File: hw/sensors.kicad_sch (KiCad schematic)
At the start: 40 parts, among them IC2 INA215CQDCKRQ1, IC5 OPA990IDCKR, IC6 INA215CQDCKRQ1, U5 MAX31865xTP, U6 ADG734

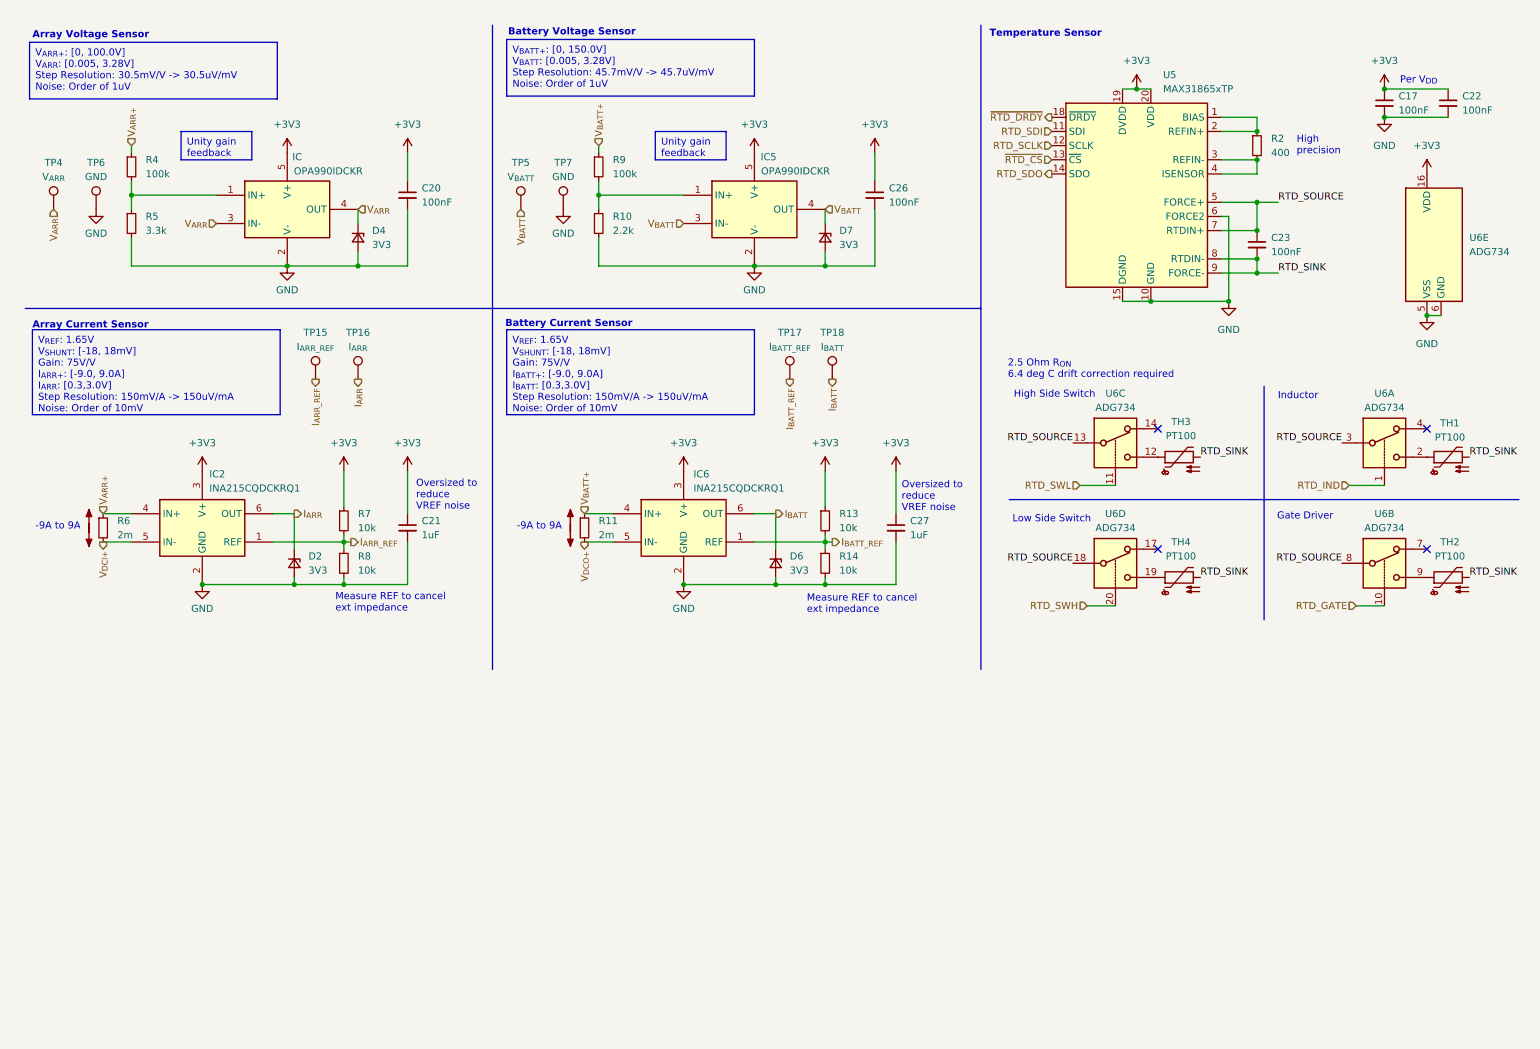
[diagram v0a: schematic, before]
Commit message: v0.3.0rc (v1.0.0rc) sch complete
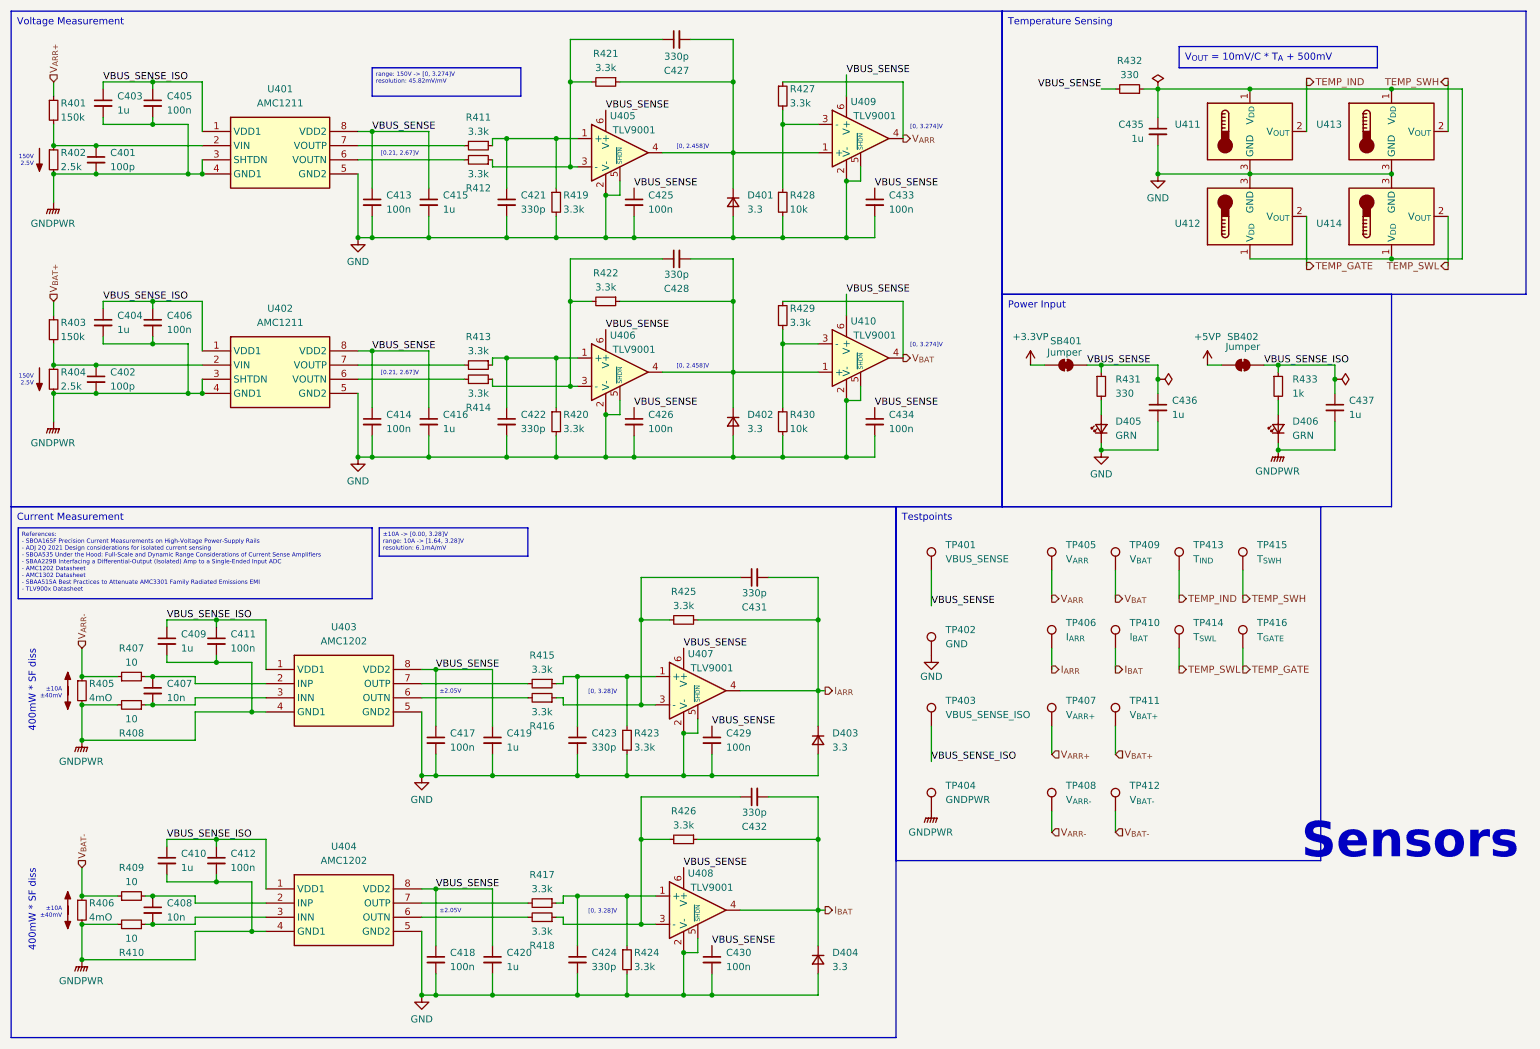
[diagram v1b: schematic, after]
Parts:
- removed C17, C20, C22, C23, C26: 100nF, symbol Device:C_Small
- removed C21, C27: 1uF, symbol Device:C_Small
- removed D2, D4, D6, D7: 3V3, Diode_SMD:D_MiniMELF, symbol Device:D_Zener_Small
- removed IC, IC5: OPA990IDCKR, footprints:ti_OPA990IDCKR, symbol ti_OPA990IDCKR:OPA990IDCKR
- removed IC2, IC6: INA215CQDCKRQ1, footprints:ti_INA215CQDCKRQ1, symbol ti_INA215CQDCKRQ1:INA215CQDCKRQ1
- removed R10: 2.2k, symbol Device:R_Small
- removed R11, R6: 2m, symbol Device:R_Small
- removed R13, R14, R7, R8: 10k, symbol Device:R_Small
- removed R2: 400, symbol Device:R_Small
- removed R4, R9: 100k, symbol Device:R_Small
- removed R5: 3.3k, symbol Device:R_Small
- removed TH1, TH2, TH3, TH4: PT100, symbol Sensor_Temperature:PT100
- removed TP15: I_{ARR_REF}, symbol Connector:TestPoint
- removed TP16: I_{ARR}, symbol Connector:TestPoint
- removed TP17: I_{BATT_REF}, symbol Connector:TestPoint
- removed TP18: I_{BATT}, symbol Connector:TestPoint
- removed TP4: V_{ARR}, symbol Connector:TestPoint
- removed TP5: V_{BATT}, symbol Connector:TestPoint
- removed TP6, TP7: GND, symbol Connector:TestPoint
- removed U5: MAX31865xTP, Package_DFN_QFN:TQFN-20-1EP_5x5mm_P0.65mm_EP3.25x3.25mm, symbol Sensor_Temperature:MAX31865xTP
- removed U6: ADG734, Package_SO:TSSOP-20_4.4x6.5mm_P0.65mm, symbol Analog_Switch:ADG734
- added C401, C402: 100p, Resistor_SMD:R_0402_1005Metric, symbol Device:C_Small
- added C403, C404, C409, C410, C415, C416, C419, C420, C435, C436, C437: 1u, Resistor_SMD:R_0402_1005Metric, symbol Device:C_Small
- added C405, C406, C411, C412, C413, C414, C417, C418, C425, C426, C429, C430, C433, C434: 100n, Resistor_SMD:R_0402_1005Metric, symbol Device:C_Small
- added C407, C408: 10n, Resistor_SMD:R_0402_1005Metric, symbol Device:C_Small
- added C421, C422, C423, C424, C427, C428, C431, C432: 330p, Resistor_SMD:R_0402_1005Metric, symbol Device:C_Small
- added D401, D402, D403, D404: 3.3, Diode_SMD:D_SOD-123, symbol Device:D_Small
- added D405, D406: GRN, LED_SMD:LED_0402_1005Metric, symbol Device:LED_Small
- added R401, R403: 150k, Resistor_SMD:R_0805_2012Metric, symbol Device:R_Small
- added R402, R404: 2.5k, Resistor_SMD:R_0805_2012Metric, symbol Device:R_Small
- added R405, R406: 4mO, Resistor_SMD:R_2512_6332Metric, symbol Device:R_Small
- added R407, R408, R409, R410: 10, Resistor_SMD:R_0402_1005Metric, symbol Device:R_Small
- added R411, R412, R413, R414, R415, R416, R417, R418, R419, R420, R421, R422, R423, R424, R425, R426, R427, R429: 3.3k, Resistor_SMD:R_0402_1005Metric, symbol Device:R_Small
- added R428, R430: 10k, Resistor_SMD:R_0402_1005Metric, symbol Device:R_Small
- added R431, R432: 330, Resistor_SMD:R_0402_1005Metric, symbol Device:R_Small
- added R433: 1k, Resistor_SMD:R_0402_1005Metric, symbol Device:R_Small
- added SB401, SB402: Jumper, Jumper:SolderJumper-2_P1.3mm_Open_TrianglePad1.0x1.5mm, symbol Jumper:SolderJumper_2_Bridged
- added TP401: VBUS_SENSE, TestPoint:TestPoint_Keystone_5000-5004_Miniature, symbol Connector:TestPoint
- added TP402: GND, TestPoint:TestPoint_Keystone_5000-5004_Miniature, symbol Connector:TestPoint
- added TP403: VBUS_SENSE_ISO, TestPoint:TestPoint_Keystone_5000-5004_Miniature, symbol Connector:TestPoint
- added TP404: GNDPWR, TestPoint:TestPoint_Keystone_5000-5004_Miniature, symbol Connector:TestPoint
- added TP405: V_{ARR}, TestPoint:TestPoint_Keystone_5000-5004_Miniature, symbol Connector:TestPoint
- added TP406: I_{ARR}, TestPoint:TestPoint_Keystone_5000-5004_Miniature, symbol Connector:TestPoint
- added TP407: V_{ARR+}, TestPoint:TestPoint_Keystone_5000-5004_Miniature, symbol Connector:TestPoint
- added TP408: V_{ARR-}, TestPoint:TestPoint_Keystone_5000-5004_Miniature, symbol Connector:TestPoint
- added TP409: V_{BAT}, TestPoint:TestPoint_Keystone_5000-5004_Miniature, symbol Connector:TestPoint
- added TP410: I_{BAT}, TestPoint:TestPoint_Keystone_5000-5004_Miniature, symbol Connector:TestPoint
- added TP411: V_{BAT+}, TestPoint:TestPoint_Keystone_5000-5004_Miniature, symbol Connector:TestPoint
- added TP412: V_{BAT-}, TestPoint:TestPoint_Keystone_5000-5004_Miniature, symbol Connector:TestPoint
- added TP413: T_{IND}, TestPoint:TestPoint_Keystone_5000-5004_Miniature, symbol Connector:TestPoint
- added TP414: T_{SWL}, TestPoint:TestPoint_Keystone_5000-5004_Miniature, symbol Connector:TestPoint
- added TP415: T_{SWH}, TestPoint:TestPoint_Keystone_5000-5004_Miniature, symbol Connector:TestPoint
- added TP416: T_{GATE}, TestPoint:TestPoint_Keystone_5000-5004_Miniature, symbol Connector:TestPoint
- added U401, U402: AMC1211, footprints:ti_AMC1211_DWV, symbol ti_AMC1211:AMC1211AQDWVRQ1
- added U403, U404: AMC1202, footprints:ti_AMC1202_DWV, symbol ti_AMC1202:AMC1202DWVR
- added U405, U406, U407, U408, U409, U410: TLV9001, Package_TO_SOT_SMD:SOT-363_SC-70-6, symbol ti_TLV9001:TLV9001
- added U411, U412, U413, U414: MCP9700A, Connector_JST:JST_PH_B3B-PH-K_1x03_P2.00mm_Vertical, symbol Sensor_Temperature:MCP9700Ax-ELT
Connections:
- net GND: now also C413.2, C414.2, C415.2, C416.2, C417.2, C418.2, C419.2, C420.2, C421.2, C422.2, C423.2, C424.2, C425.2, C426.2, C429.2, C430.2, C433.2, C434.2, C435.2, C436.2, D401.2 (A), D402.2 (A), D403.2 (A), D404.2 (A), D405.1 (K), R419.2, R420.2, R423.2, R424.2, R428.2, R430.2, TP402.1, U401.5 (GND2), U402.5 (GND2), U403.5 (GND2), U404.5 (GND2), U405.2 (V-), U405.5 (~{SHDN}), U406.2 (V-), U406.5 (~{SHDN}), U407.2 (V-), U407.5 (~{SHDN}), U408.2 (V-), U408.5 (~{SHDN}), U409.2 (V-), U409.5 (~{SHDN}), U410.2 (V-), U410.5 (~{SHDN}), U411.3 (GND), U412.3 (GND), U413.3 (GND), U414.3 (GND)
- net I_{ARR}: now also C431.2, D403.1 (K), R425.1, TP406.1, U407.4
- net V_{ARR+}: now also R401.1, TP407.1
- net V_{ARR}: now also R427.1, TP405.1, U409.4
- new net: C424.1, R417.1, R424.1, U408.1 (+)
- new net: C432.1, R418.1, R426.2, U408.3 (-)
- new net: C423.1, R415.1, R423.1, U407.1 (+)
- new net: C431.1, R416.1, R425.2, U407.3 (-)
- new net: C428.1, R414.1, R422.2, U406.3 (-)
- new net: R414.2, U402.6 (VOUTN)
- new net: C407.2, R408.1, U403.3 (INN)
- new net: R416.2, U403.6 (OUTN)
- new net: C427.2, D401.1 (K), R421.1, U405.4, U409.1 (+)
- new net: C421.1, R411.1, R419.1, U405.1 (+)
- new net: D406.2 (A), R433.2
- new net: C428.2, D402.1 (K), R422.1, U406.4, U410.1 (+)
- new net: R429.2, R430.1, U410.3 (-)
- new net: C402.1, R403.2, R404.1, U402.2 (VIN)
- new net: C427.1, R412.1, R421.2, U405.3 (-)
- new net: C407.1, R407.2, U403.2 (INP)
- new net: R415.2, U403.7 (OUTP)
- new net: C422.1, R413.1, R420.1, U406.1 (+)
- new net: D405.2 (A), R431.2
- new net: R427.2, R428.1, U409.3 (-)
- new net: C408.2, R410.1, U404.3 (INN)
- new net: C401.1, R401.2, R402.1, U401.2 (VIN)
- new net: R418.2, U404.6 (OUTN)
- new net: C435.1, R432.1, U411.1 (V_{DD}), U412.1 (V_{DD}), U413.1 (V_{DD}), U414.1 (V_{DD})
- new net: R413.2, U402.7 (VOUTP)
- new net: C408.1, R409.2, U404.2 (INP)
- new net: R417.2, U404.7 (OUTP)
- new net: R412.2, U401.6 (VOUTN)
- new net: R411.2, U401.7 (VOUTP)
- new net +3.3VP: SB401.1 (A)
- new net +5VP: SB402.1 (A)
- new net GNDPWR: C401.2, C402.2, C403.2, C404.2, C405.2, C406.2, C409.2, C410.2, C411.2, C412.2, C437.2, D406.1 (K), R402.2, R404.2, R405.2, R406.2, R408.2, R410.2, TP404.1, U401.3 (SHTDN), U401.4 (GND1), U402.3 (SHTDN), U402.4 (GND1), U403.4 (GND1), U404.4 (GND1)
- new net I_{BAT}: C432.2, D404.1 (K), R426.1, TP410.1, U408.4
- new net TEMP_GATE: TP416.1, U412.2 (V_{OUT})
- new net TEMP_IND: TP413.1, U411.2 (V_{OUT})
- new net TEMP_SWH: TP415.1, U413.2 (V_{OUT})
- new net TEMP_SWL: TP414.1, U414.2 (V_{OUT})
- new net VBUS_SENSE: C413.1, C414.1, C415.1, C416.1, C417.1, C418.1, C419.1, C420.1, C425.1, C426.1, C429.1, C430.1, C433.1, C434.1, C436.1, R431.1, R432.2, SB401.2 (B), TP401.1, U401.8 (VDD2), U402.8 (VDD2), U403.8 (VDD2), U404.8 (VDD2), U405.6 (V+), U406.6 (V+), U407.6 (V+), U408.6 (V+), U409.6 (V+), U410.6 (V+)
- new net VBUS_SENSE_ISO: C403.1, C404.1, C405.1, C406.1, C409.1, C410.1, C411.1, C412.1, C437.1, R433.1, SB402.2 (B), TP403.1, U401.1 (VDD1), U402.1 (VDD1), U403.1 (VDD1), U404.1 (VDD1)
- new net V_{ARR-}: R405.1, R407.1, TP408.1
- new net V_{BAT+}: R403.1, TP411.1
- new net V_{BAT-}: R406.1, R409.1, TP412.1
- new net V_{BAT}: R429.1, TP409.1, U410.4
- no-connect marks 4 -> 0
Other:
- note added: "150V 2.5V"
- note added: "400mW * SF diss"
- note added: "Sensors"
- note added: "[0, 2.458]V"
- note added: "[0, 3.274]V"
- note added: "[0, 3.28]V"
- note added: "[0.21, 2.67]V"
- note added: "±10A ±40mV"
- note added: "±2.05V"
- note removed: "-9A to 9A"
- note removed: "2.5 Ohm R_{ON} 6.4 deg C drift correction required"
- note removed: "Array Current Sensor"
- note removed: "Array Voltage Sensor"
- note removed: "Battery Current Sensor"
- note removed: "Battery Voltage Sensor"
- note removed: "Gate Driver"
- note removed: "High Side Switch"
- note removed: "High precision"
- note removed: "Inductor"
- note removed: "Low Side Switch"
- note removed: "Measure REF to cancel ext impedance"
- note removed: "Oversized to reduce VREF noise"
- note removed: "Per V_{DD}"
- note removed: "Temperature Sensor"
